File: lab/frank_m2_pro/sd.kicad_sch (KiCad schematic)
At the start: 2 parts, among them J13 104031-0811

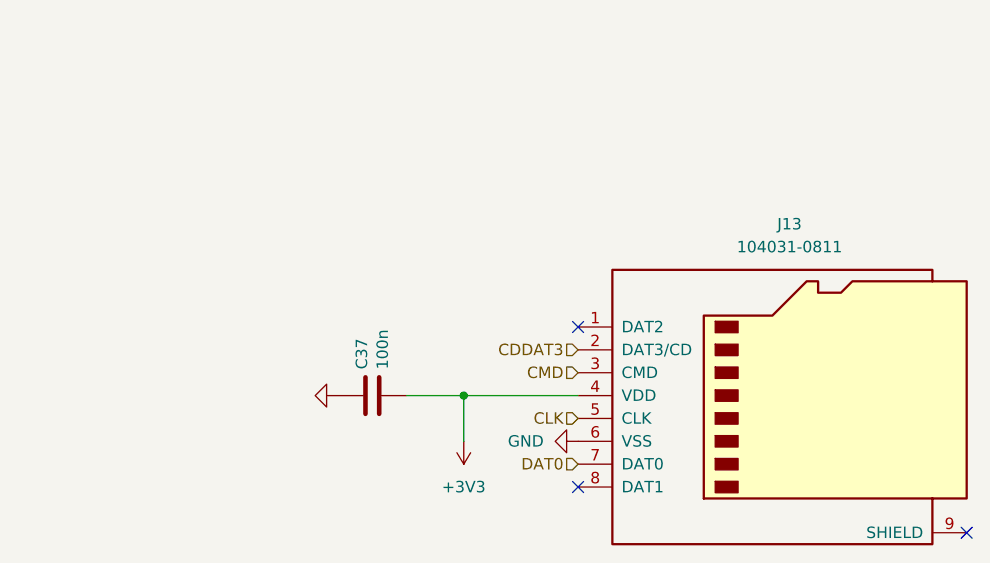
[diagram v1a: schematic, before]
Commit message: FRANK M1 Pro HW 1.00
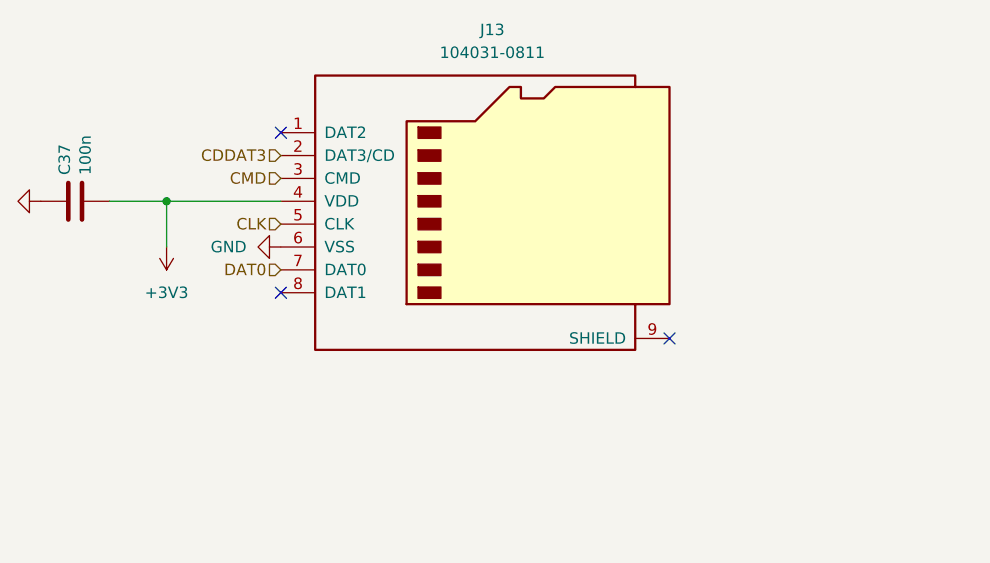
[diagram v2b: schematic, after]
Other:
- moved on the sheet: C37, J13
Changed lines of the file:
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@@
 		(rev "${VERSION}")
 		(company "Mikhail Matveev")
-		(comment 1 "https://github.com/xtremespb/frank")
+		(comment 1 "https://github.com/rh1tech/frank")
 	)
 	(junction
-		(at 162.56 115.57)
+		(at 129.54 93.98)
 		(diameter 0)
 		(color 0 0 0 0)
 	)
 	(no_connect
-		(at 218.44 130.81)
+		(at 185.42 109.22)
 	)
 	(no_connect
-		(at 175.26 125.73)
+		(at 142.24 104.14)
 	)
 	(no_connect
-		(at 175.26 107.95)
+		(at 142.24 86.36)
 	)
 	(wire
 		(pts
-			(xy 162.56 115.57) (xy 156.21 115.57)
+			(xy 129.54 93.98) (xy 123.19 93.98)
 		)
 		(stroke
@@
 	(wire
 		(pts
-			(xy 162.56 115.57) (xy 175.26 115.57)
+			(xy 129.54 93.98) (xy 142.24 93.98)
 		)
 		(stroke
@@
 	(wire
 		(pts
-			(xy 162.56 120.65) (xy 162.56 115.57)
+			(xy 129.54 99.06) (xy 129.54 93.98)
 		)
 		(stroke
@@
 	(hierarchical_label "CMD"
 		(shape input)
-		(at 175.26 113.03 180)
+		(at 142.24 91.44 180)
 		(effects
 			(font
@@
 	(hierarchical_label "DAT0"
 		(shape input)
-		(at 175.26 123.19 180)
+		(at 142.24 101.6 180)
 		(effects
 			(font
@@
 	(hierarchical_label "CDDAT3"
 		(shape input)
-		(at 175.26 110.49 180)
+		(at 142.24 88.9 180)
 		(effects
 			(font
@@
 	(hierarchical_label "CLK"
 		(shape input)
-		(at 175.26 118.11 180)
+		(at 142.24 96.52 180)
 		(effects
 			(font
@@
 	(symbol
 		(lib_id "FRANK:C")
-		(at 152.4 115.57 90)
+		(at 119.38 93.98 90)
 		(unit 1)
 		(exclude_from_sim no)
@@
 		(dnp no)
 		(property "Reference" "C37"
-			(at 151.2316 112.649 0)
+			(at 118.2116 91.059 0)
 			(effects
 				(font
@@
 		)
 		(property "Value" "100n"
-			(at 153.543 112.649 0)
+			(at 120.523 91.059 0)
 			(effects
 				(font
@@
 		)
 		(property "Footprint" "FRANK:C_0805_2012Metric"
-			(at 156.21 114.6048 0)
+			(at 123.19 93.0148 0)
 			(effects
 				(font
@@
 		)
 		(property "Datasheet" "~"
-			(at 152.4 115.57 0)
+			(at 119.38 93.98 0)
 			(effects
 				(font
@@
 		)
 		(property "Description" "Unpolarized capacitor"
-			(at 152.4 115.57 0)
+			(at 119.38 93.98 0)
 			(effects
 				(font
@@
 		)
 		(property "AliExpress" "https://www.aliexpress.com/item/33008008276.html"
-			(at 152.4 115.57 0)
+			(at 119.38 93.98 0)
 			(effects
 				(font
@@
 	(symbol
 		(lib_id "power:+3V3")
-		(at 162.56 120.65 180)
+		(at 129.54 99.06 180)
 		(unit 1)
 		(exclude_from_sim no)
@@
 		(fields_autoplaced yes)
 		(property "Reference" "#PWR0129"
-			(at 162.56 116.84 0)
+			(at 129.54 95.25 0)
 			(effects
 				(font
@@
 		)
 		(property "Value" "+3V3"
-			(at 162.56 125.73 0)
+			(at 129.54 104.14 0)
 			(effects
 				(font
@@
 		)
 		(property "Footprint" ""
-			(at 162.56 120.65 0)
+			(at 129.54 99.06 0)
 			(effects
 				(font
@@
 		)
 		(property "Datasheet" ""
-			(at 162.56 120.65 0)
+			(at 129.54 99.06 0)
 			(effects
 				(font
@@
 		)
 		(property "Description" "Power symbol creates a global label with name \"+3V3\""
-			(at 162.56 120.65 0)
+			(at 129.54 99.06 0)
 			(effects
 				(font
@@
 	(symbol
 		(lib_id "power:GND")
-		(at 148.59 115.57 270)
+		(at 115.57 93.98 270)
 		(unit 1)
 		(exclude_from_sim no)
@@
 		(dnp no)
 		(property "Reference" "#PWR0128"
-			(at 142.24 115.57 0)
+			(at 109.22 93.98 0)
 			(effects
 				(font
@@
 		)
 		(property "Value" "GND"
-			(at 146.05 121.92 0)
+			(at 113.03 100.33 0)
 			(effects
 				(font
@@
 		)
 		(property "Footprint" ""
-			(at 148.59 115.57 0)
+			(at 115.57 93.98 0)
 			(effects
 				(font
@@
 		)
 		(property "Datasheet" ""
-			(at 148.59 115.57 0)
+			(at 115.57 93.98 0)
 			(effects
 				(font
@@
 		)
 		(property "Description" "Power symbol creates a global label with name \"GND\" , ground"
-			(at 148.59 115.57 0)
+			(at 115.57 93.98 0)
 			(effects
 				(font
@@
 	(symbol
 		(lib_id "power:GND")
-		(at 175.26 120.65 270)
+		(at 142.24 99.06 270)
 		(unit 1)
 		(exclude_from_sim no)
@@
 		(fields_autoplaced yes)
 		(property "Reference" "#PWR0130"
-			(at 168.91 120.65 0)
+			(at 135.89 99.06 0)
 			(effects
 				(font
@@
 		)
 		(property "Value" "GND"
-			(at 171.45 120.6499 90)
+			(at 138.43 99.0599 90)
 			(effects
 				(font
@@
 		)
 		(property "Footprint" ""
-			(at 175.26 120.65 0)
+			(at 142.24 99.06 0)
 			(effects
 				(font
@@
 		)
 		(property "Datasheet" ""
-			(at 175.26 120.65 0)
+			(at 142.24 99.06 0)
 			(effects
 				(font
@@
 		)
 		(property "Description" "Power symbol creates a global label with name \"GND\" , ground"
-			(at 175.26 120.65 0)
+			(at 142.24 99.06 0)
 			(effects
 				(font
@@
 	(symbol
 		(lib_id "Connector:Micro_SD_Card")
-		(at 198.12 115.57 0)
+		(at 165.1 93.98 0)
 		(unit 1)
 		(exclude_from_sim no)
@@
 		(fields_autoplaced yes)
 		(property "Reference" "J13"
-			(at 198.755 96.52 0)
+			(at 165.735 74.93 0)
 			(effects
 				(font
@@
 		)
 		(property "Value" "104031-0811"
-			(at 198.755 99.06 0)
+			(at 165.735 77.47 0)
 			(effects
 				(font
@@
 		)
 		(property "Footprint" "FRANK:MicroSD (SMD, long)"
-			(at 227.33 107.95 0)
+			(at 194.31 86.36 0)
 			(effects
 				(font
@@
 		)
 		(property "Datasheet" "https://www.we-online.com/components/products/datasheet/693072010801.pdf"
-			(at 198.12 115.57 0)
+			(at 165.1 93.98 0)
 			(effects
 				(font
@@
 		)
 		(property "Description" "Micro SD Card Socket"
-			(at 198.12 115.57 0)
+			(at 165.1 93.98 0)
 			(effects
 				(font
@@
 		)
 		(property "AliExpress" "https://www.aliexpress.com/item/1005004214252441.html"
-			(at 198.12 115.57 0)
-			(effects
-				(font
+			(at 165.1 93.98 0)
+			(effects
+				(font
